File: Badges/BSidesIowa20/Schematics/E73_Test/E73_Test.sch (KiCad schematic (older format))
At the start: 27 parts, among them J1 Conn_01x02, J2 Oled, J4 Conn_02x04_Odd_Even, J7 USB_C_Receptacle, SW2 SW_DIP_x01, SW4 SW_DIP_x01, U2 TLV1117-33, U3 HX4056, U5 K1-5202UA-03(5Way_Switch)

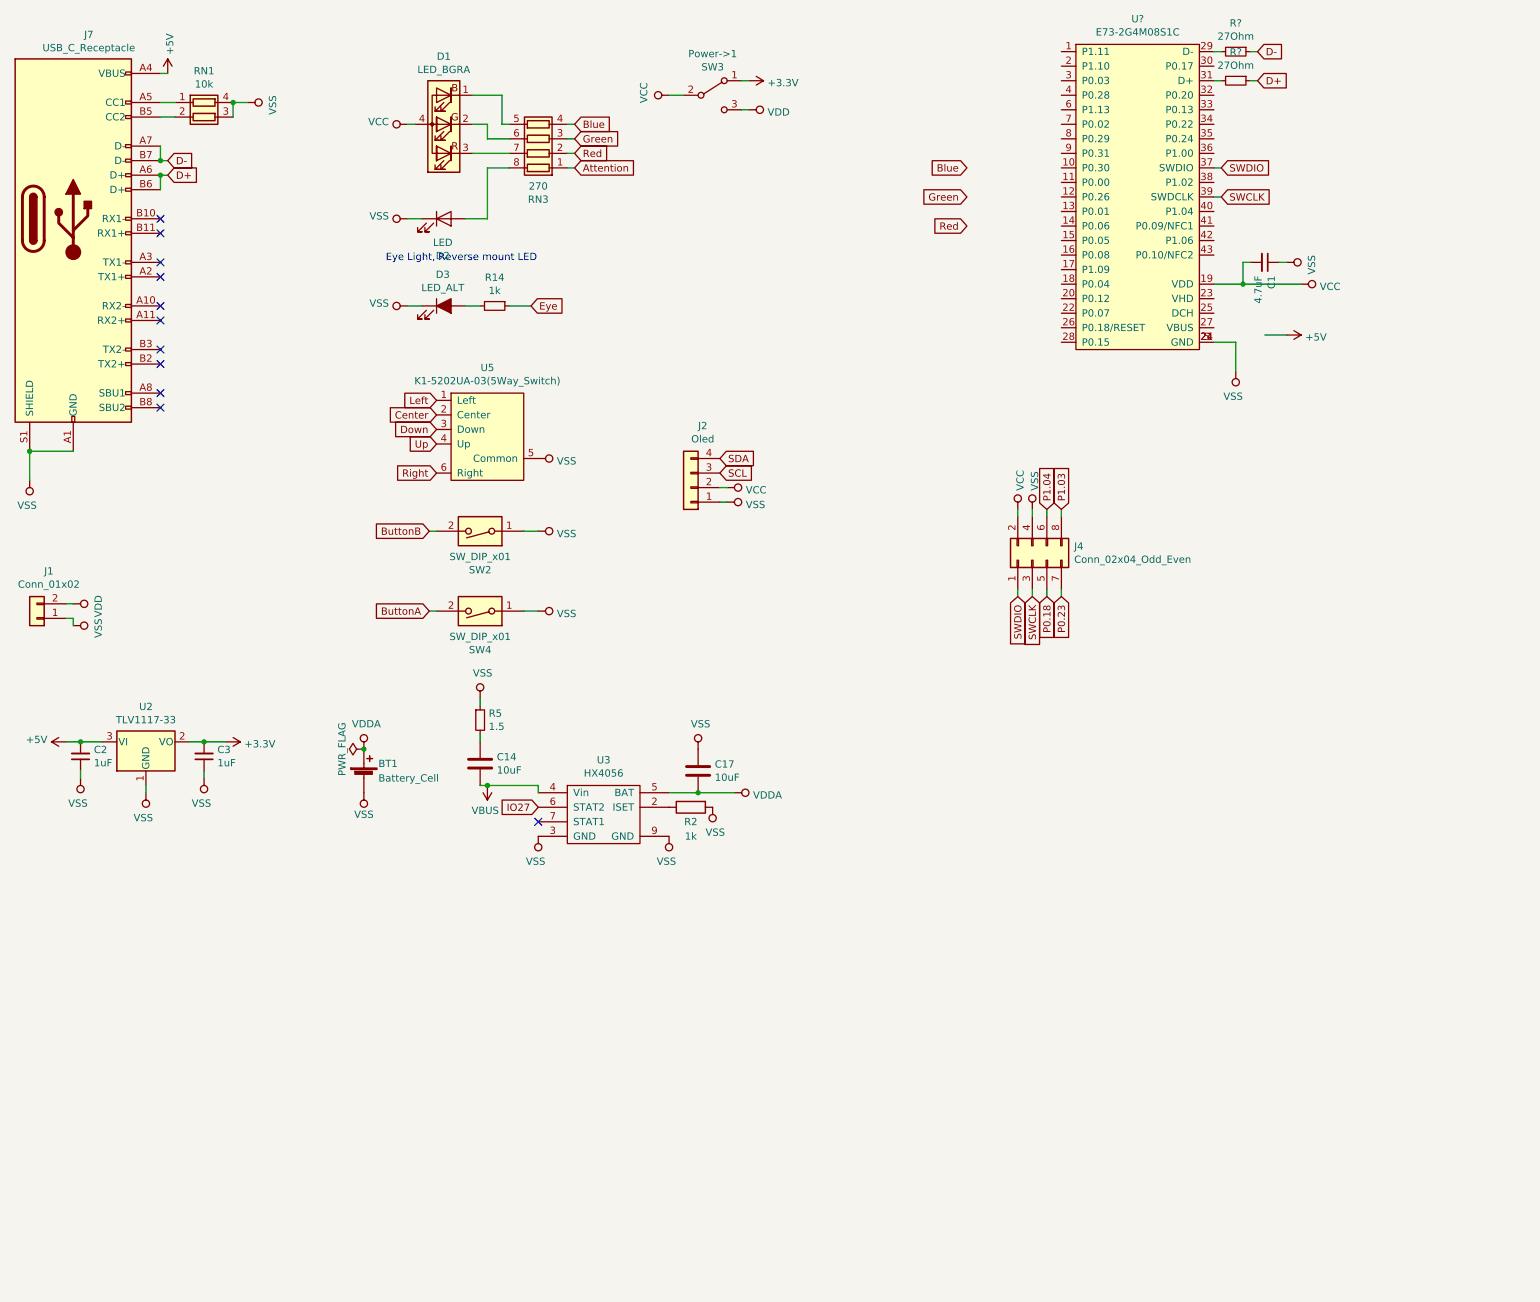
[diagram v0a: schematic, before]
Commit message: Putting stuff together
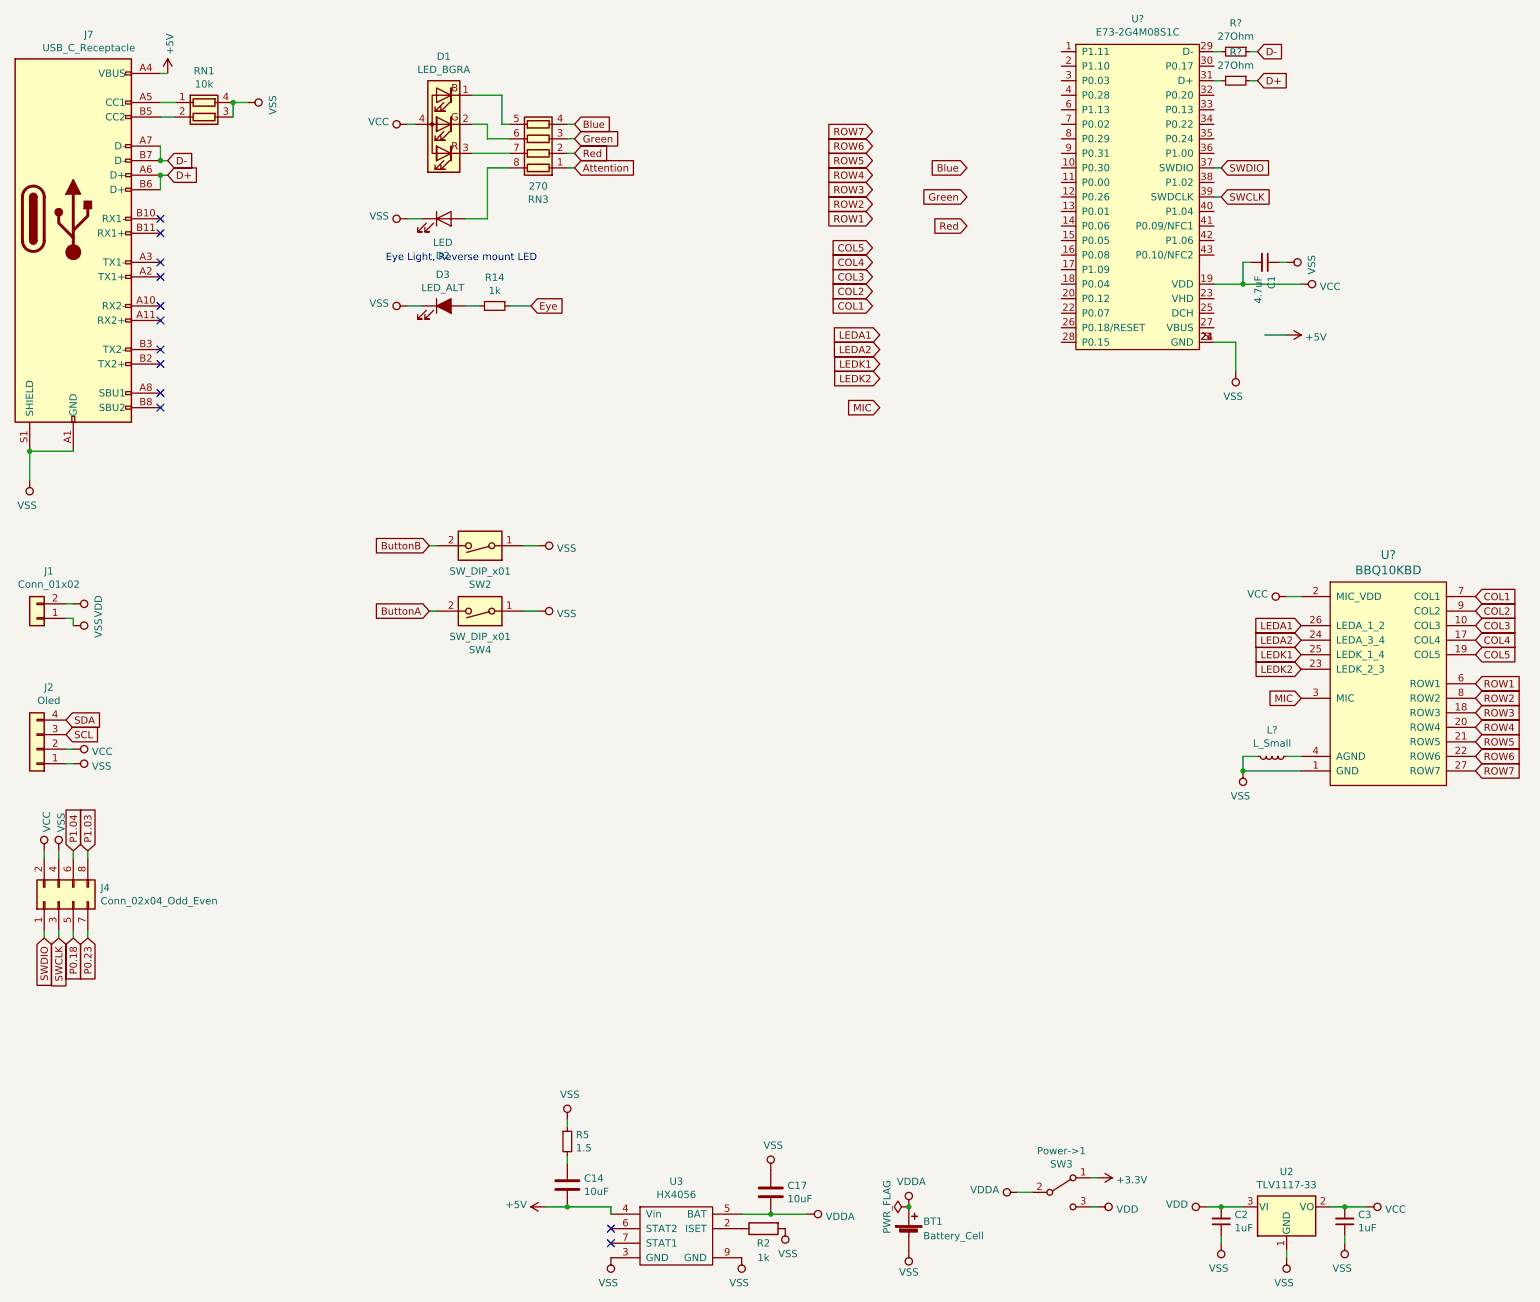
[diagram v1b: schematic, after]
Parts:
- removed U5: K1-5202UA-03(5Way_Switch), Dragos:K1-5202UA-03(5way-switch), symbol dragos-rescue:K1-5202UA-03(5Way_Switch)-Dragos
- added L?: L_Small, symbol Device:L_Small
- added U?: BBQ10KBD, symbol Keyboard:BBQ10KBD
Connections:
- net VBUS is gone; now on net +5V: C14.2, U3.4 (Vin)
- net +3V3: no longer C3.2, U2.2 (VO)
- net +5V: no longer C2.2, U2.3 (VI)
- net VCC: now also C3.2, U2.2 (VO), U?.2 (MIC_VDD); no longer Power->1.2 (B)
- net VDD: now also C2.2, U2.3 (VI)
- net VDDA: now also Power->1.2 (B)
- net VSS: now also L?.2, U?.1 (GND), U?.11 (GND), U?.12 (GND), U?.13 (GND), U?.14 (GND), U?.15 (GND), U?.16 (GND), U?.28 (GND), U?.5 (GND)
- net IO27: no longer names the net of U3.6 (STAT2)
- new net: L?.1, U?.4 (AGND)
- new net COL1: U?.7 (COL1)
- new net COL2: U?.9 (COL2)
- new net COL3: U?.10 (COL3)
- new net COL4: U?.17 (COL4)
- new net COL5: U?.19 (COL5)
- new net LEDA1: U?.26 (LEDA_1_2)
- new net LEDA2: U?.24 (LEDA_3_4)
- new net LEDK1: U?.25 (LEDK_1_4)
- new net LEDK2: U?.23 (LEDK_2_3)
- new net MIC: U?.3 (MIC)
- new net ROW1: U?.6 (ROW1)
- new net ROW2: U?.8 (ROW2)
- new net ROW3: U?.18 (ROW3)
- new net ROW4: U?.20 (ROW4)
- new net ROW5: U?.21 (ROW5)
- new net ROW6: U?.22 (ROW6)
- new net ROW7: U?.27 (ROW7)
- no-connect marks 11 -> 12
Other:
- moved on the sheet: BT1, C14, C17, C2, C3, J2, J4, Power->1, R2, R5, SW2, U2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
